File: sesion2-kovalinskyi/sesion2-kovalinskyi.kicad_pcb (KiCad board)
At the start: 4 copper layers, 64.5 x 35.7 mm, 36 parts, among them J1 Screw_Terminal_01x02, J2 Conn_01x06_Pin, J3 USB_C_Receptacle_USB2.0_16P, SW1 SW_Push, U1 LD1117S33TR_SOT223, U2 ATmega328P-AU, U3 MCP9808, U4 ADXL343, U6 CH340C

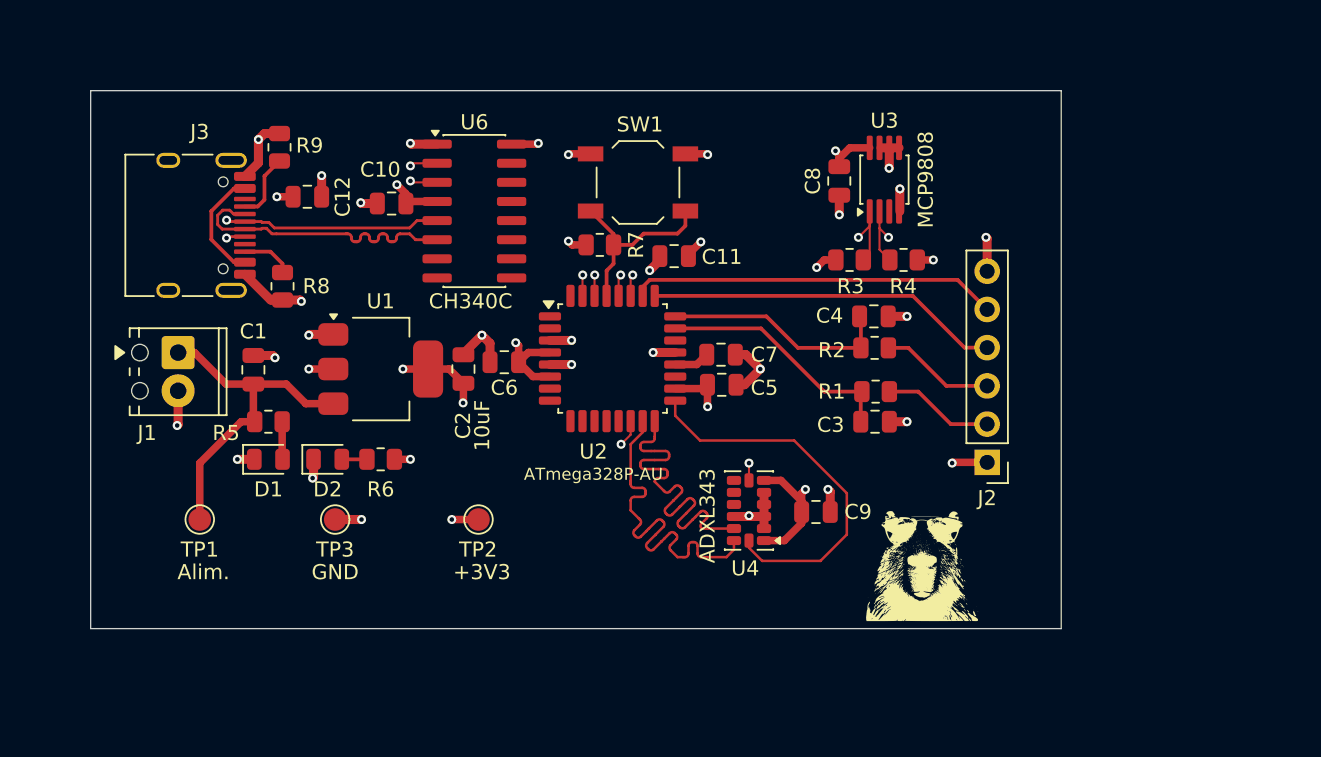
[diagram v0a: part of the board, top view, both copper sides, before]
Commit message: Sesión 5 - LAYOUT FINAL (verificar Vías de Cosido)
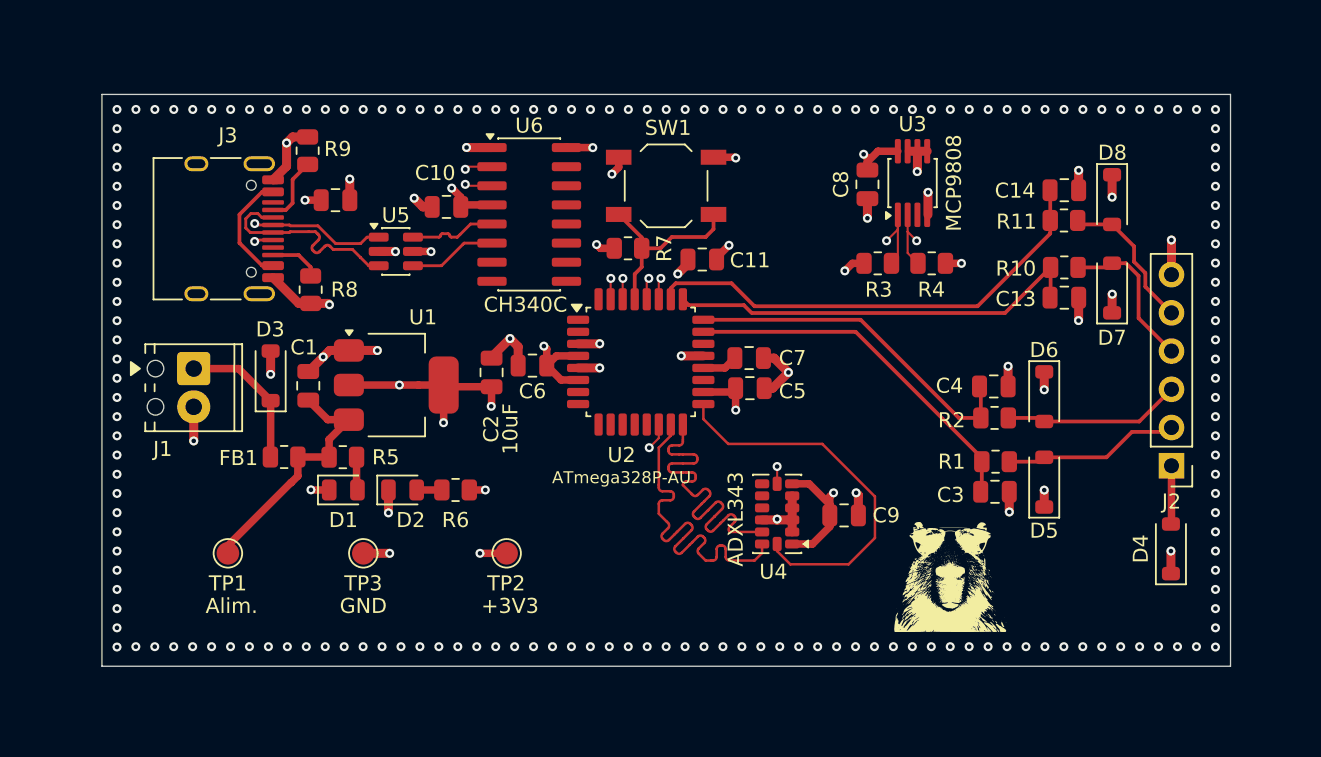
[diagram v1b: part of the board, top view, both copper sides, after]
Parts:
- added C13: 100nF, Capacitor_SMD:C_0805_2012Metric, F.Cu at (164.0, 103.5)
- added C14: 100nF, Capacitor_SMD:C_0805_2012Metric, F.Cu at (164.0, 96.4)
- added D3: D_TVS, Diode_SMD:D_SOD-123, F.Cu at (111.2, 108.7)
- added D4: D_TVS, Diode_SMD:D_SOD-123, F.Cu at (171.0, 120.2)
- added D5: D_TVS, Diode_SMD:D_SOD-123, F.Cu at (162.6, 115.8)
- added D6: D_TVS, Diode_SMD:D_SOD-123, F.Cu at (162.6, 110.1)
- added D7: D_TVS, Diode_SMD:D_SOD-123, F.Cu at (167.1, 102.9)
- added D8: D_TVS, Diode_SMD:D_SOD-123, F.Cu at (167.1, 97.0)
- added FB1: 100 Ohm @ 100MHz, Resistor_SMD:R_0805_2012Metric, F.Cu at (112.1, 114.1)
- added R10: 1k, Resistor_SMD:R_0805_2012Metric, F.Cu at (164.0, 101.5)
- added R11: 1k, Resistor_SMD:R_0805_2012Metric, F.Cu at (163.9, 98.4)
- added U5: USBLC6-2SC6, Package_TO_SOT_SMD:SOT-23-6, F.Cu at (119.5, 100.4)
- moved J2 12.3 mm to (171.1, 114.7)
- moved C3 9.23 mm to (159.3, 116.4)
- moved C4 9.23 mm to (159.3, 109.4)
- moved R1 9.23 mm to (159.4, 114.4)
- moved R2 9.23 mm to (159.3, 111.5)
- moved R5 5.48 mm to (116.0, 114.1)
- moved D1 5.38 mm to (116.0, 116.3)
- moved D2 5.38 mm to (120.0, 116.3)
- moved R6 5.38 mm to (123.5, 116.3)
- moved C1 3.80 mm to (113.7, 109.4)
- moved U6 3.65 mm to (128.4, 98.0)
- moved C10 3.65 mm to (122.9, 97.5)
- moved TP1 2.92 mm to (108.4, 120.5)
- moved TP2 2.92 mm to (126.9, 120.5)
- moved TP3 2.92 mm to (117.4, 120.5)
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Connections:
- C1 pad 2: Net-(J1-Pin_1) -> Net-(U1-VI)
- J1 pad 1: Net-(J1-Pin_1) -> Net-(D3-A1)
- J2 pad 4: Net-(J2-Pin_4) -> Net-(D7-A2)
- J2 pad 5: Net-(J2-Pin_5) -> Net-(D8-A2)
- J3 pad A6: /UART-USB/USB+ -> /UART-USB/C_USB+
- J3 pad A7: /UART-USB/USB- -> /UART-USB/C_USB-
- J3 pad B6: /UART-USB/USB+ -> /UART-USB/C_USB+
- J3 pad B7: /UART-USB/USB- -> /UART-USB/C_USB-
- R5 pad 2: Net-(J1-Pin_1) -> Net-(U1-VI)
- TP1 pad 1: Net-(J1-Pin_1) -> Net-(U1-VI)
- U1 pad 3: Net-(J1-Pin_1) -> Net-(U1-VI)
- U2 pad 25: Net-(J2-Pin_4) -> /microcontrolador/PIN_25
- U2 pad 26: Net-(J2-Pin_5) -> /microcontrolador/PIN_26
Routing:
- net /microcontrolador/PIN_26: track 0.00 -> 31.6 mm
- net /microcontrolador/PIN_25: track 0.00 -> 28.1 mm
- net Net-(J2-Pin_5): track 24.5 -> 0.00 mm
- net Net-(J2-Pin_4): track 23.5 -> 0.00 mm
- net Net-(J1-Pin_1): track 22.8 -> 0.00 mm
- net Net-(U1-VI): track 0.00 -> 16.7 mm
- net /UART-USB/GND: track 55.6 -> 70.3 mm, vias 27 -> 208
- net /UART-USB/C_USB-: track 0.00 -> 14.1 mm
- net /UART-USB/USB-: track 19.6 -> 5.87 mm
- net /UART-USB/C_USB+: track 0.00 -> 11.4 mm, vias 0 -> 2
- net /UART-USB/USB+: track 16.9 -> 5.86 mm, vias 2 -> 0
- net Net-(D7-A2): track 0.00 -> 10.4 mm
- net Net-(D8-A2): track 0.00 -> 9.91 mm
- net Net-(D3-A1): track 0.00 -> 9.75 mm
- net /UART-USB/+3V3: track 47.2 -> 56.0 mm
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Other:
- board size 64.5 x 35.7 mm -> 75 x 38 mm
